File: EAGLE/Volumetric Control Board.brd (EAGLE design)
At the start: 160 x 100 mm, 2 parts, among them U2 SN74HCT125NG4

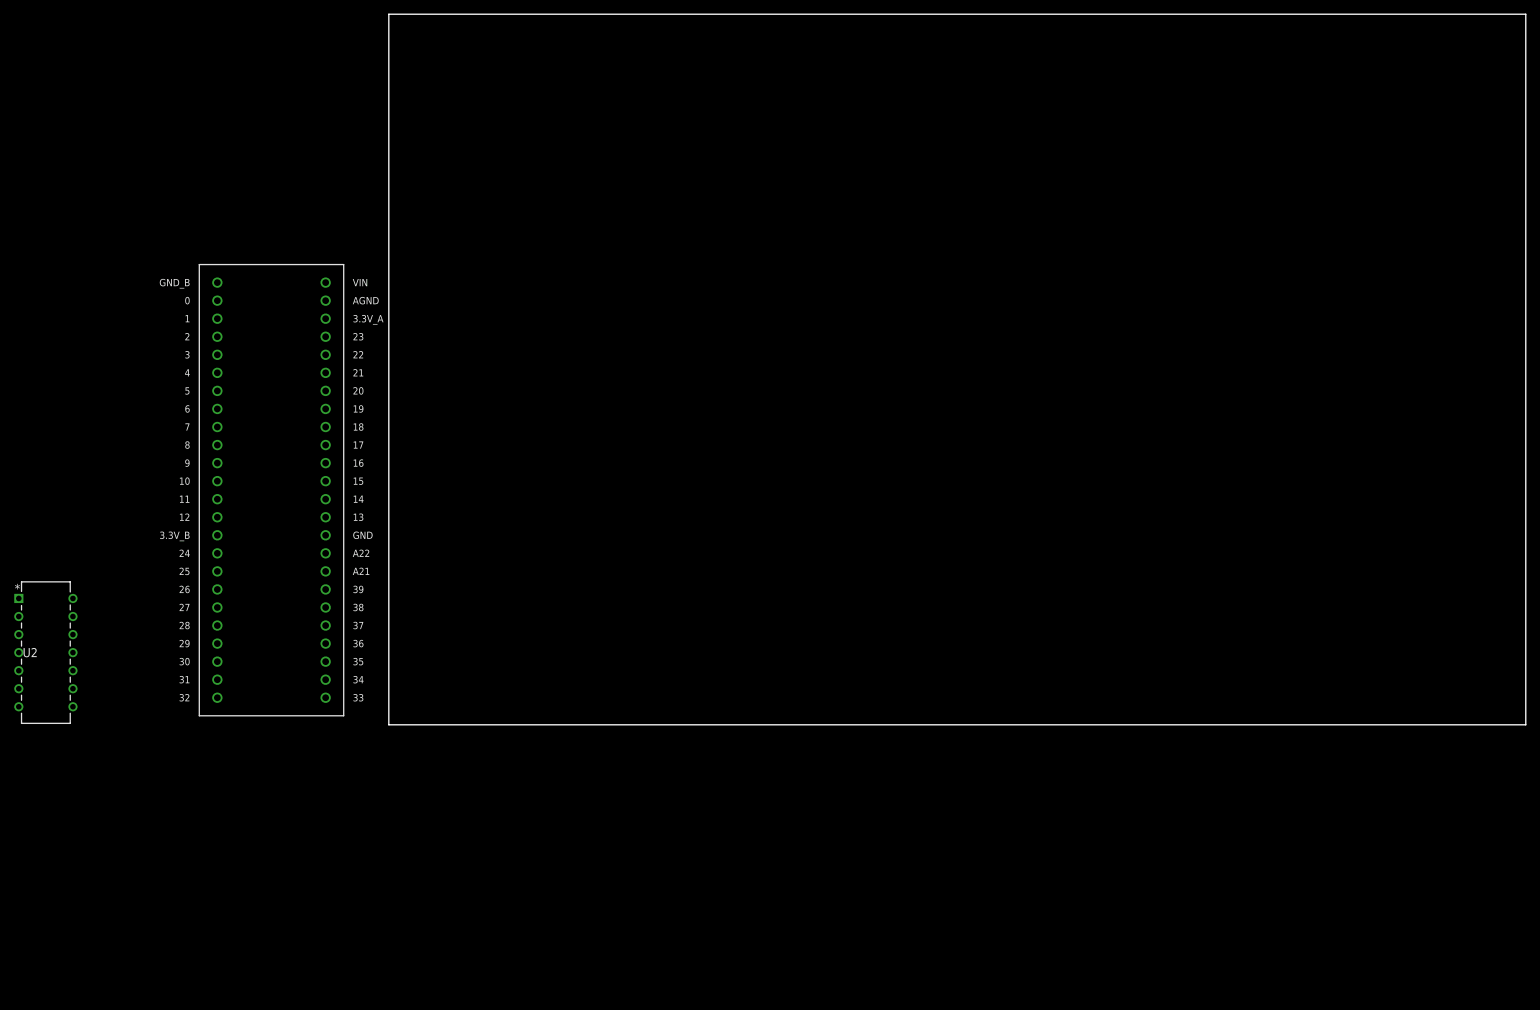
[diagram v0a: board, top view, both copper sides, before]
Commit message: adsf
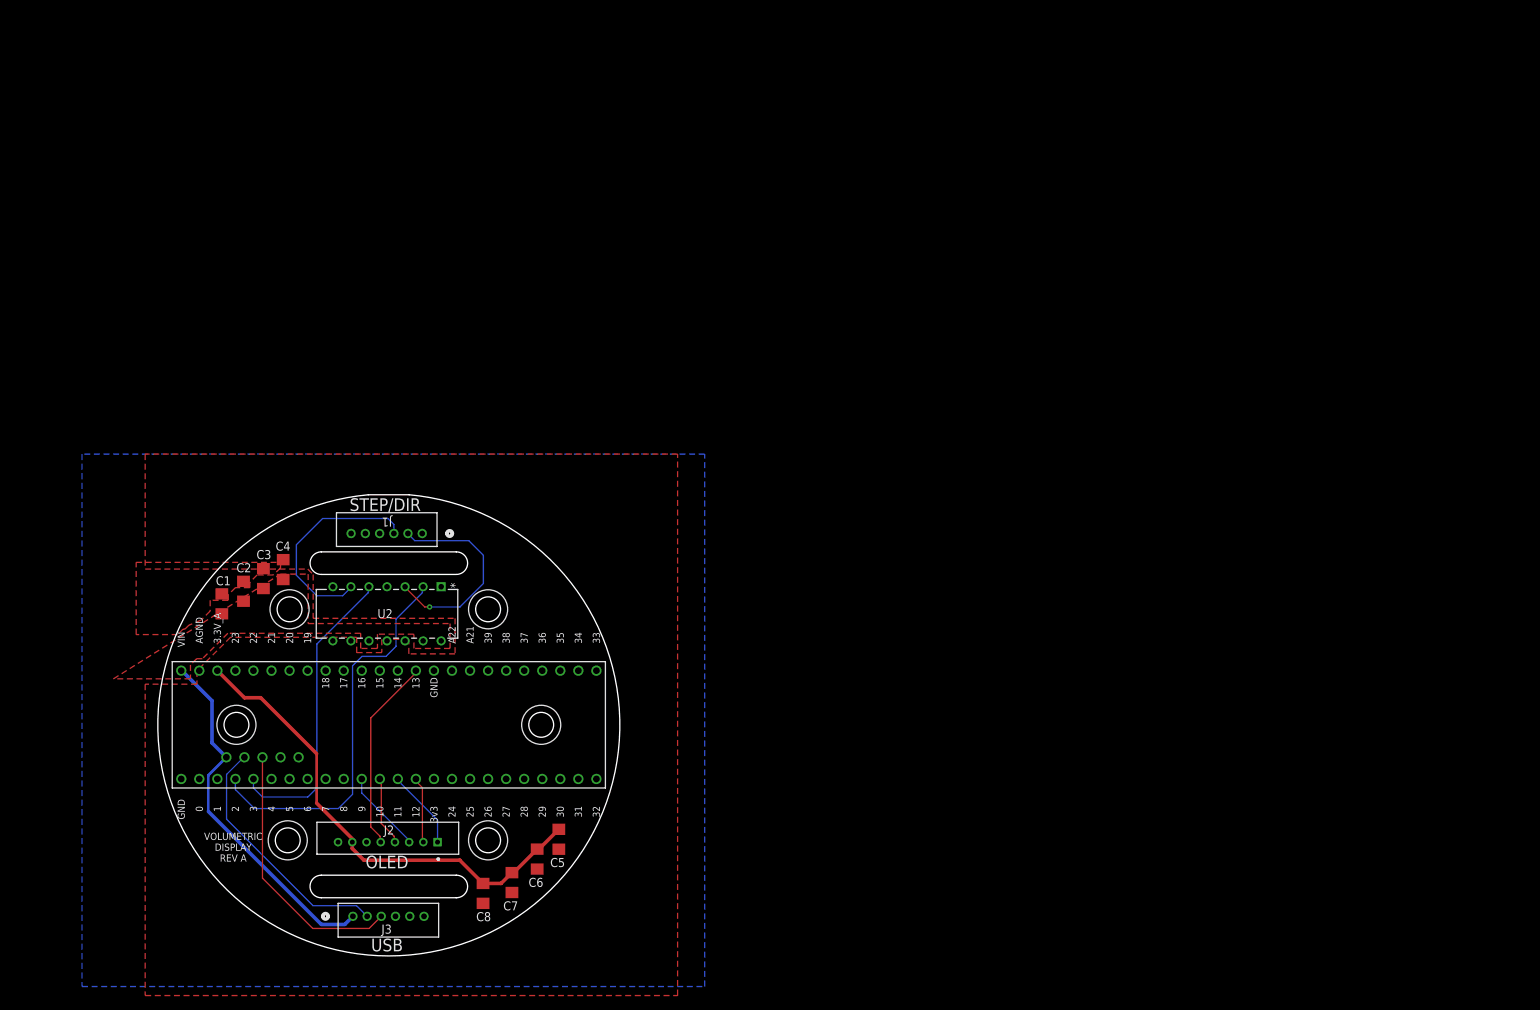
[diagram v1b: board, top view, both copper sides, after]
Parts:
- added C1, C5: 10uF, rcl:C1206
- added C2, C6: 1uF, rcl:C1206
- added C3, C7: 0.1uF, rcl:C1206
- added C4, C8: 0.01uF, rcl:C1206
- added J1, J3: B6B-PH-K-S(LF)(SN), volumetric_display:CONN_B6B-PH-K-S_JST
- added J2: B8B-PH-K-S(LF)(SN), volumetric_display:JST_B8B-PH-K-S(LF)(SN)
- moved U2 59.5 mm to (7.37, 19.4), turned to 270 degrees
- moved U$1 58.3 mm to (-29.2, 7.62), turned to 90 degrees
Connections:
- new net 3.3V: C5.1, C6.1, C7.1, C8.1, J2.7, U$1.3.3V_A
- new net CS: J2.3, U$1.9
- new net D/C: J2.4, U$1.10
- new net MISO: J2.2, U$1.12
- new net MOSI: J2.1, U$1.11
- new net SCLK: J2.5, U$1.13
- new net USB_DM: J3.2, U$1.USB_DM
- new net USB_DP: J3.3, U$1.USB_DP
- net 5V: now also C1.1, C2.1, C3.1, C4.1, J3.1, U$1.USB_5V
- net DIR_5V: now also J1.3
- net GND: now also C1.2, C2.2, C3.2, C4.2, C5.2, C6.2, C7.2, C8.2, J1.4, J2.6, J3.4, U$1.USB_GND, U$1.USB_GND2
- net STEP_5V: now also J1.2
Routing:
- net 3.3V: track 0.00 -> 68.7 mm
- net STEP: track 0.00 -> 55.2 mm
- net 5V: track 0.00 -> 51.2 mm
- net DIR: track 0.00 -> 42.6 mm
- net USB_DP: track 0.00 -> 37.4 mm
- net USB_DM: track 0.00 -> 35.3 mm
- net DIR_5V: track 0.00 -> 30.6 mm
- net STEP_5V: track 0.00 -> 29.5 mm, vias 0 -> 1
- net SCLK: track 0.00 -> 27.3 mm
- net CS: track 0.00 -> 11.7 mm
- net MOSI: track 0.00 -> 11.3 mm
- net D/C: track 0.00 -> 9.82 mm
- net MISO: track 0.00 -> 9.36 mm
- added copper zone on layer 1, net 5V
- added copper zone on layer 1, net GND
- added copper zone on layer 16, net GND
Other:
- board size 160 x 100 mm -> 65 x 64.9 mm
- board text added: "OLED"
- board text added: "STEP/DIR"
- board text added: "USB"
- board text added: "VOLUMETRIC DISPLAY REV A"
